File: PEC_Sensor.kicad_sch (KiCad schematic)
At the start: 47 parts, among them IC1 TC4420, J1 Conn_01x03_Pin, J2 Conn_01x03_Pin, J3 Conn_01x02_Pin, J4 Conn_01x02_Pin, J5 Conn_01x02_Pin, J6 Conn_01x02_Pin, J7 Conn_01x02_Pin, J8 Conn_01x02_Pin, Q1 SSM3K336R, U1 AD8221, U2 OPA820, U3 TPS54331

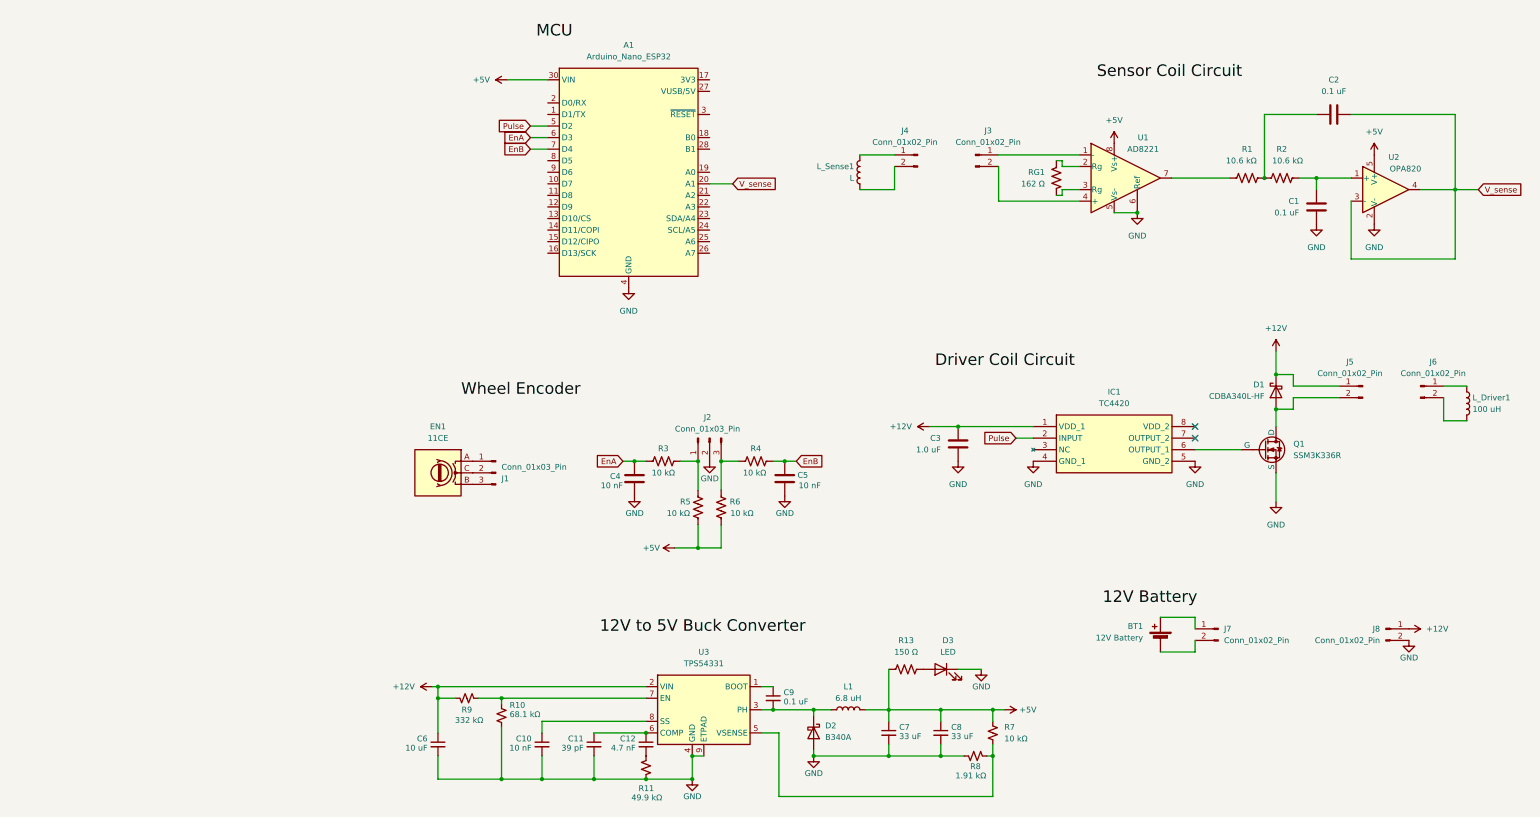
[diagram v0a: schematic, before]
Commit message: jan 29
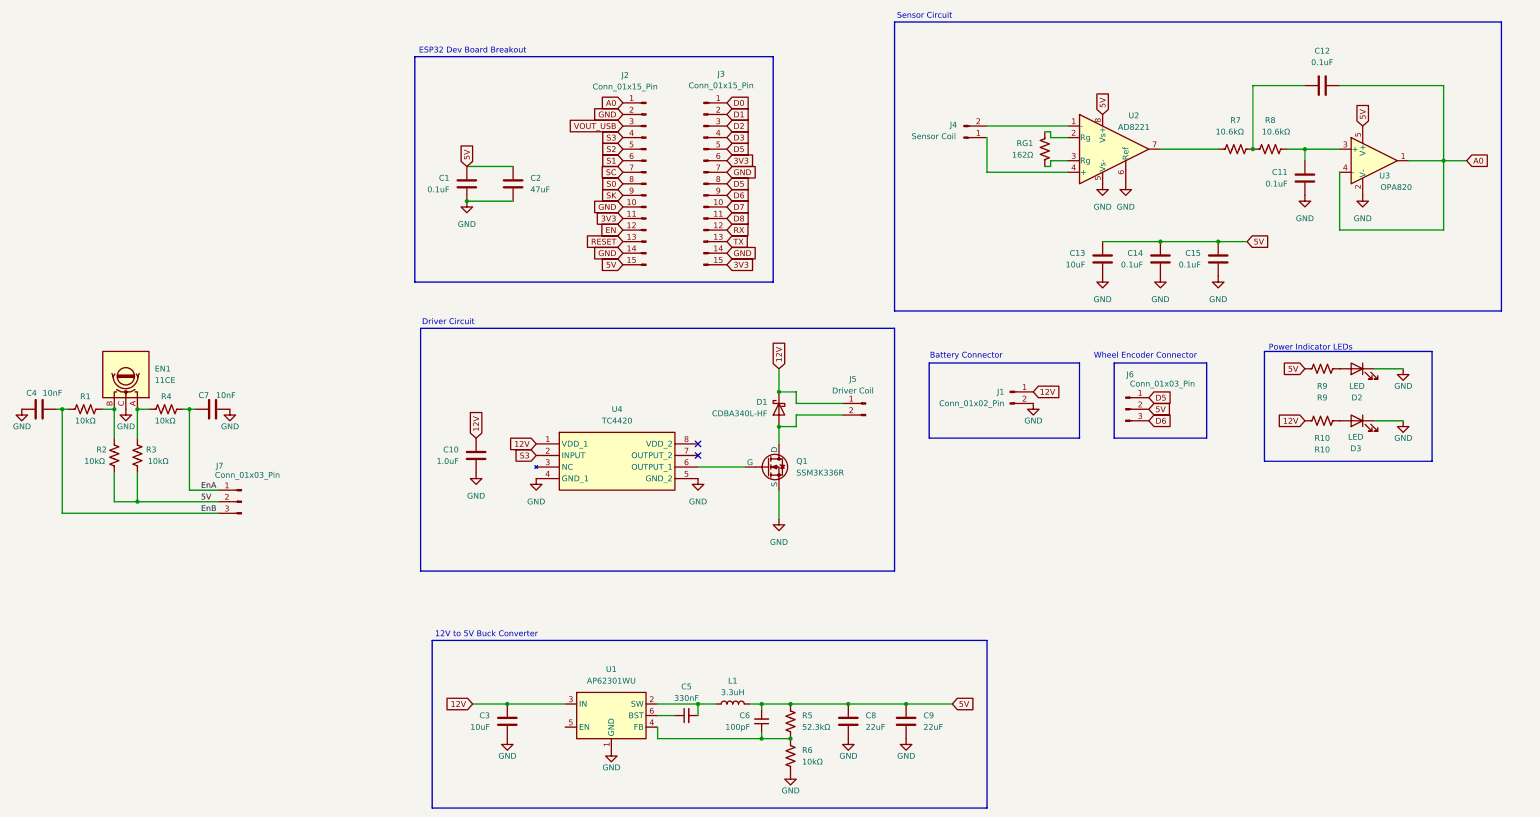
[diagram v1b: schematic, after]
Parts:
- removed A1: Arduino_Nano_ESP32, RF_Module:ESP32-C6-MINI-1, symbol MCU_Module:Arduino_Nano_ESP32
- removed BT1: 12V Battery, symbol Device:Battery_Cell
- removed C10: 10 nF, symbol Device:C_Small
- removed C11: 39 pF, symbol Device:C_Small
- removed C12: 4.7 nF, symbol Device:C_Small
- removed C7, C8: 33 uF, symbol Device:C_Small
- removed C9: 0.1 uF, symbol Device:C_Small
- removed D2: B340A, symbol Device:D_Schottky
- removed J1: Conn_01x03_Pin, Connector_JST:JST_EH_S3B-EH_1x03_P2.50mm_Horizontal, symbol Connector:Conn_01x03_Pin
- removed J4, J6, J7: Conn_01x02_Pin, symbol Connector:Conn_01x02_Pin
- removed L_Driver1: 100 uH, symbol Device:L
- removed L_Sense1: L, symbol Device:L
- removed R10: 68.1 kΩ, symbol Device:R_Small_US
- removed R11: 49.9 kΩ, symbol Device:R_Small_US
- removed R13: 150 Ω, symbol Device:R_US
- removed R7: 10 kΩ, symbol Device:R_Small_US
- removed R8: 1.91 kΩ, symbol Device:R_Small_US
- removed R9: 332 kΩ, symbol Device:R_Small_US
- removed U3: TPS54331, Package_SO:HVSSOP-10-1EP_3x3mm_P0.5mm_EP1.57x1.88mm_ThermalVias, symbol Regulator_Switching:TPS54336ADDA
- added C1: 0.1uF, symbol Device:C
- added C13: 10uF, Capacitor_SMD:C_0603_1608Metric, symbol Device:C
- added C14, C15: 0.1uF, Capacitor_SMD:C_0603_1608Metric, symbol Device:C
- added C2: 47uF, symbol Device:C
- added C3: 10uF, symbol Device:C
- added C5: 330nF, symbol Device:C_Small
- added C8, C9: 22uF, symbol Device:C
- added D2: LED, symbol Device:LED
- added J2, J3: Conn_01x15_Pin, Connector_PinHeader_2.54mm:PinHeader_1x15_P2.54mm_Vertical, symbol Connector:Conn_01x15_Pin
- added J6: Conn_01x03_Pin, symbol Connector:Conn_01x03_Pin
- added R10: R10, symbol Device:R_US
- added R5: 52.3kΩ, symbol Device:R_US
- added R6: 10kΩ, symbol Device:R_US
- added R9: R9, symbol Device:R_US
- added U1: AP62301WU, Package_TO_SOT_SMD:TSOT-23-6, symbol Regulator_Switching:AP62301WU
- C10: renamed from C3; value 1.0 uF -> 1.0uF; footprint (none) -> Capacitor_SMD:C_0603_1608Metric
- C11: renamed from C1; value 0.1 uF -> 0.1uF; footprint (none) -> Capacitor_SMD:C_0603_1608Metric
- C12: renamed from C2; value 0.1 uF -> 0.1uF; footprint (none) -> Capacitor_SMD:C_0603_1608Metric
- C4: value 10 nF -> 10nF
- C6: value 10 uF -> 100pF
- C7: renamed from C5; value 10 nF -> 10nF
- D1: footprint Diode_SMD:D_SMA -> (none)
- J1: renamed from J8; footprint (none) -> Connector_BarrelJack:BarrelJack_Horizontal
- J4: renamed from J3; value Conn_01x02_Pin -> Sensor Coil; footprint (none) -> Connector_JST:JST_EH_S2B-EH_1x02_P2.50mm_Horizontal
- J5: value Conn_01x02_Pin -> Driver Coil; footprint (none) -> Connector_JST:JST_EH_S2B-EH_1x02_P2.50mm_Horizontal
- J7: renamed from J2; footprint Connector_JST:JST_EH_S3B-EH_1x03_P2.50mm_Horizontal -> (none)
- L1: value 6.8 uH -> 3.3uH; footprint (none) -> Inductor_SMD:L_Taiyo-Yuden_NR-50xx
- R1: renamed from R3; value 10 kΩ -> 10kΩ
- R2: renamed from R5; value 10 kΩ -> 10kΩ
- R3: renamed from R6; value 10 kΩ -> 10kΩ
- R4: value 10 kΩ -> 10kΩ
- R7: renamed from R1; value 10.6 kΩ -> 10.6kΩ; footprint (none) -> Resistor_SMD:R_0603_1608Metric
- R8: renamed from R2; value 10.6 kΩ -> 10.6kΩ; footprint (none) -> Resistor_SMD:R_0603_1608Metric
- RG1: value 162 Ω -> 162Ω; footprint Resistor_SMD:R_01005_0402Metric_Pad0.57x0.30mm_HandSolder -> Resistor_SMD:R_0603_1608Metric
- U3: renamed from U2; footprint Package_TO_SOT_SMD:SOT-353_SC-70-5 -> Package_TO_SOT_SMD:SOT-23-5
- renumbered U1 to U2, IC1 to U4
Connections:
- net EnA: now also C7.1, J7.1 (Pin_1), R4.1; no longer C4.1, R1.2
- net EnB: now also C4.2, J7.3 (Pin_3), R1.2; no longer C7.1, R4.1
- net GND: now also C4.1, EN1.C, C1.2, C13.1, C14.1, C15.1, C2.2, C3.2, C8.2, C9.2, D2.1 (K), J2.10 (Pin_10), J2.14 (Pin_14), J2.2 (Pin_2), J3.14 (Pin_14), J3.7 (Pin_7), R6.2, U1.1 (GND); no longer C4.2, C6.2, J7.2 (Pin_2)
- net at J4.1 (Pin_1): now also U2.4 (+); no longer U2.1 (-)
- net at J4.2 (Pin_2): now also U2.1 (-); no longer U2.4 (+)
- net at L1.1: now also C5.2, U1.2 (SW)
- net at D3.2 (A): now also R10.2
- net at EN1.A: now also R3.1, R4.2
- net at EN1.B: now also R1.1, R2.1
- net at C11.1, R8.1: now also U3.3 (+); no longer U3.1 (+)
- net +12V renamed 12V
- net 12V: now also C3.1, R10.1, U1.3 (IN); no longer C6.1
- net +5V renamed 5V
- net 5V: now also C6.2, J7.2 (Pin_2), C1.1, C13.2, C14.2, C15.2, C2.1, C8.1, C9.1, J2.15 (Pin_15), J6.2 (Pin_2), R5.1, R9.1
- net Pulse renamed S3
- net S3: now also J2.4 (Pin_4)
- net V_sense renamed A0
- net A0: now also U3.1, J2.1 (Pin_1); no longer U3.3 (-)
- new net: D2.2 (A), R9.2
- new net: C6.1, R5.2, R6.1, U1.4 (FB)
- new net: C5.1, U1.6 (BST)
- new net 3V3: J2.11 (Pin_11), J3.15 (Pin_15), J3.6 (Pin_6)
- new net D0: J3.1 (Pin_1)
- new net D1: J3.2 (Pin_2)
- new net D2: J3.3 (Pin_3)
- new net D3: J3.4 (Pin_4)
- new net D5: J3.5 (Pin_5), J3.8 (Pin_8), J6.1 (Pin_1)
- new net D6: J3.9 (Pin_9), J6.3 (Pin_3)
- new net D7: J3.10 (Pin_10)
- new net D8: J3.11 (Pin_11)
- new net EN: J2.12 (Pin_12)
- new net RESET: J2.13 (Pin_13)
- new net RX: J3.12 (Pin_12)
- new net S0: J2.8 (Pin_8)
- new net S1: J2.6 (Pin_6)
- new net S2: J2.5 (Pin_5)
- new net SC: J2.7 (Pin_7)
- new net SK: J2.9 (Pin_9)
- new net TX: J3.13 (Pin_13)
- new net VOUT_USB: J2.3 (Pin_3)
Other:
- note added: "12V to 5V Buck Converter"
- note added: "Battery Connector"
- note added: "Driver Circuit"
- note added: "ESP32 Dev Board Breakout"
- note added: "Power Indicator LEDs"
- note added: "Sensor Circuit"
- note added: "Wheel Encoder Connector"
- moved on the sheet: C10, C11, C12, C4, C7, D1, EN1, J1, J4, J5, J7, Q1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
